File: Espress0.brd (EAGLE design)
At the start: 36.8 x 39.4 mm, 41 parts, among them CN1 4U#20329, Q2 reset, U1 AP2112K-3.3, U2 2MB Flash, U3 MCP73831T-2ACI/OT

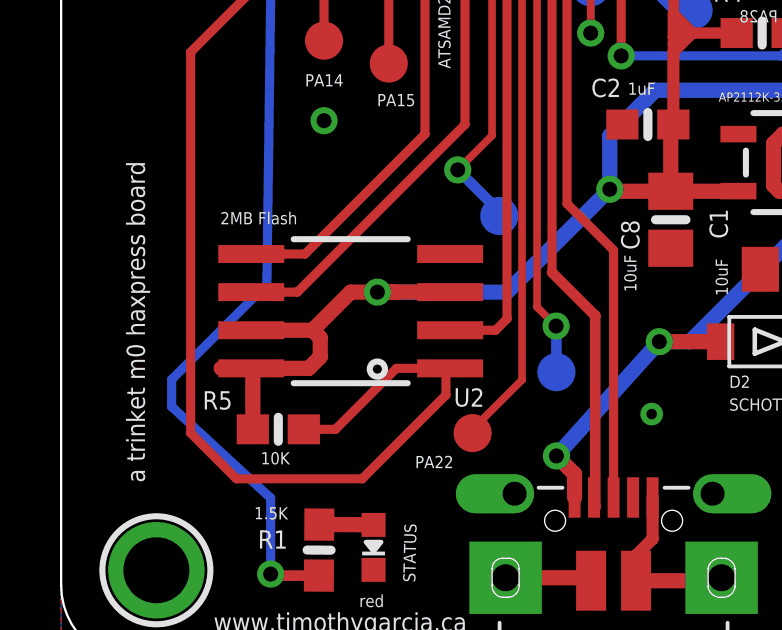
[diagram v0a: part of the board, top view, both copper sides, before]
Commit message: Add files via upload
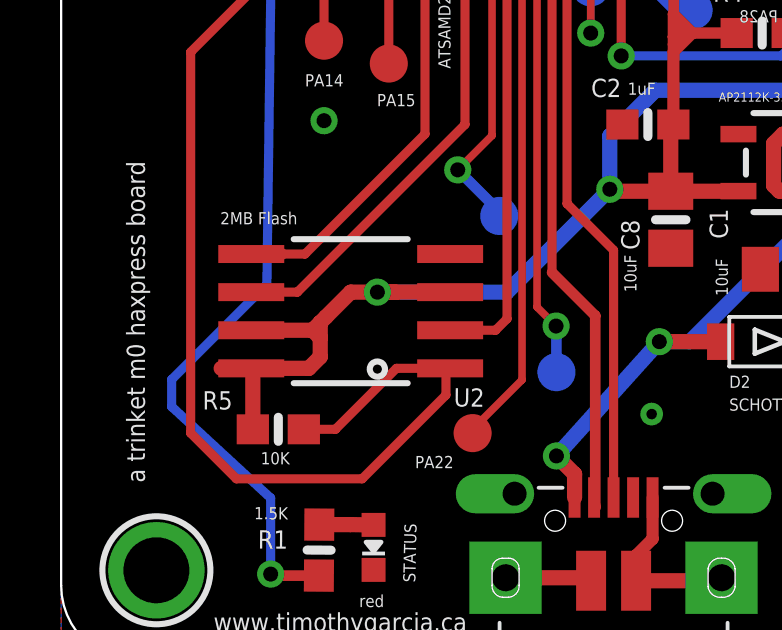
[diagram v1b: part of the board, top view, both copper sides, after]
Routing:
- net 3.3V: track 101.4 -> 101.9 mm
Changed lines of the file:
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@@
 <wire x1="19.0897875" y1="35.4727875" x2="19.0897875" y2="31.6399" width="0.508" layer="16"/>
 <wire x1="6.337" y1="11.049" x2="8.382" y2="11.049" width="0.508" layer="1"/>
-<wire x1="8.382" y1="11.049" x2="8.636" y2="10.795" width="0.508" layer="1"/>
+<wire x1="8.636" y1="10.795" x2="8.382" y2="11.049" width="0.508" layer="1"/>
 <wire x1="8.636" y1="10.795" x2="8.636" y2="10.16" width="0.508" layer="1"/>
 <wire x1="8.636" y1="10.16" x2="8.255" y2="9.779" width="0.508" layer="1"/>
@@
 <wire x1="16.5735" y1="25.5905" x2="18.034" y2="24.13" width="0.508" layer="16"/>
 <wire x1="18.034" y1="24.13" x2="20.447" y2="24.13" width="0.508" layer="16"/>
-<wire x1="8.382" y1="11.049" x2="9.652" y2="12.319" width="0.508" layer="1"/>
+<wire x1="8.382" y1="11.049" x2="8.636" y2="11.303" width="0.508" layer="1"/>
+<wire x1="8.636" y1="11.303" x2="8.8265" y2="11.4935" width="0.508" layer="1"/>
+<wire x1="8.8265" y1="11.4935" x2="9.652" y2="12.319" width="0.508" layer="1"/>
 <wire x1="9.652" y1="12.319" x2="10.541" y2="12.319" width="0.508" layer="1"/>
+<wire x1="8.636" y1="10.795" x2="8.636" y2="11.303" width="0.508" layer="1"/>
 </signal>
 <signal name="D1_A0_PA02">
